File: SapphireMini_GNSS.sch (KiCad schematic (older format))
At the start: 13 parts, among them J701 Conn_01x04_Male, J702 Conn_01x01_Male, J703 Conn_01x06_Male, U701 TPS22860DBVR

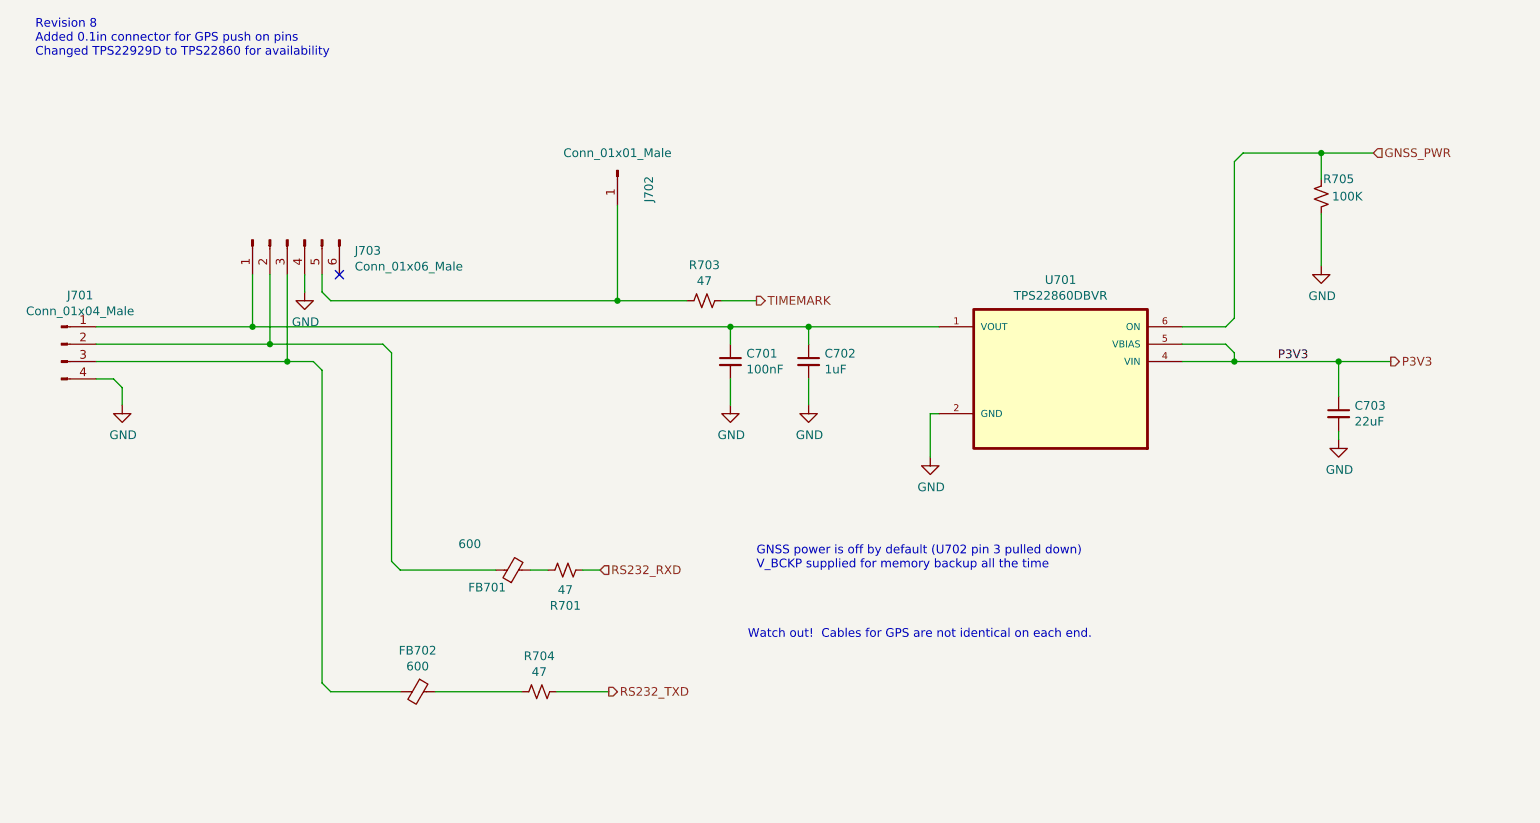
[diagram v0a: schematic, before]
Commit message: From RA_Old Modified"
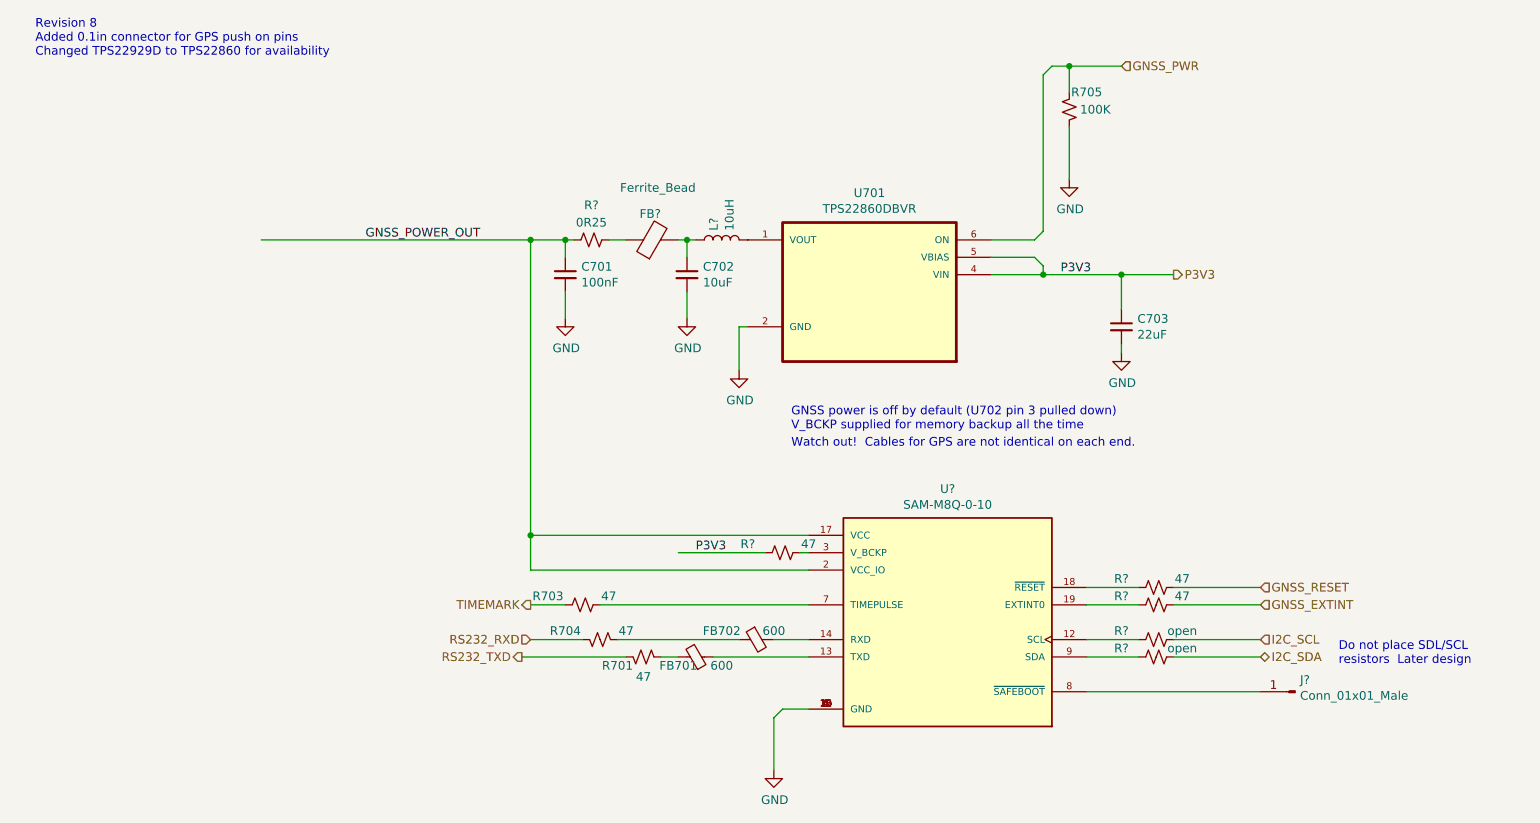
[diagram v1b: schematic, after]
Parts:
- removed J701: Conn_01x04_Male, Connector_JST:JST_SH_SM04B-SRSS-TB_1x04-1MP_P1.00mm_Horizontal, symbol Connector:Conn_01x04_Male
- removed J702: Conn_01x01_Male, Connector_PinHeader_1.27mm:PinHeader_1x01_P1.27mm_Vertical, symbol Connector:Conn_01x01_Male
- removed J703: Conn_01x06_Male, Connector_PinHeader_2.54mm:PinHeader_1x06_P2.54mm_Horizontal, symbol Connector:Conn_01x06_Male
- added FB?: Ferrite_Bead, symbol Device:Ferrite_Bead
- added J?: Conn_01x01_Male, symbol Connector:Conn_01x01_Male
- added L?: 10uH, symbol Device:L
- added R? (x3): 47, Resistor_SMD:R_0603_1608Metric, symbol Device:R_Small_US
- added R? (x2): open, Resistor_SMD:R_0603_1608Metric, symbol Device:R_Small_US
- added R?: 0R25, Resistor_SMD:R_0603_1608Metric, symbol Device:R_Small_US
- added U?: SAM-M8Q-0-10, MODULE_SAM-M8Q-0-10, symbol sapphireMini:SAM-M8Q-0-10
- C702: value 1uF -> 10uF
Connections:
- net labels added: GNSS_EXTINT, GNSS_POWER_OUT, GNSS_RESET, I2C_SCL, I2C_SDA
- wire segments 55 -> 54
- no-connect marks 1 -> 0
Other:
- note added: "Do not place SDL/SCL\nresistors Later design"
- moved on the sheet: C701, C702, C703, FB701, FB702, R701, R703, R704, R705, U701
